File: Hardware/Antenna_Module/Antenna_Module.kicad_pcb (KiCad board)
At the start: 2 copper layers, 80 x 80 mm, 18 parts, among them J1 Conn_Coaxial, J2 Conn_01x02_Pin, U1 X3C14P1-03S-1, U2 X3C14P1-03S-1, U3 TFM.120A

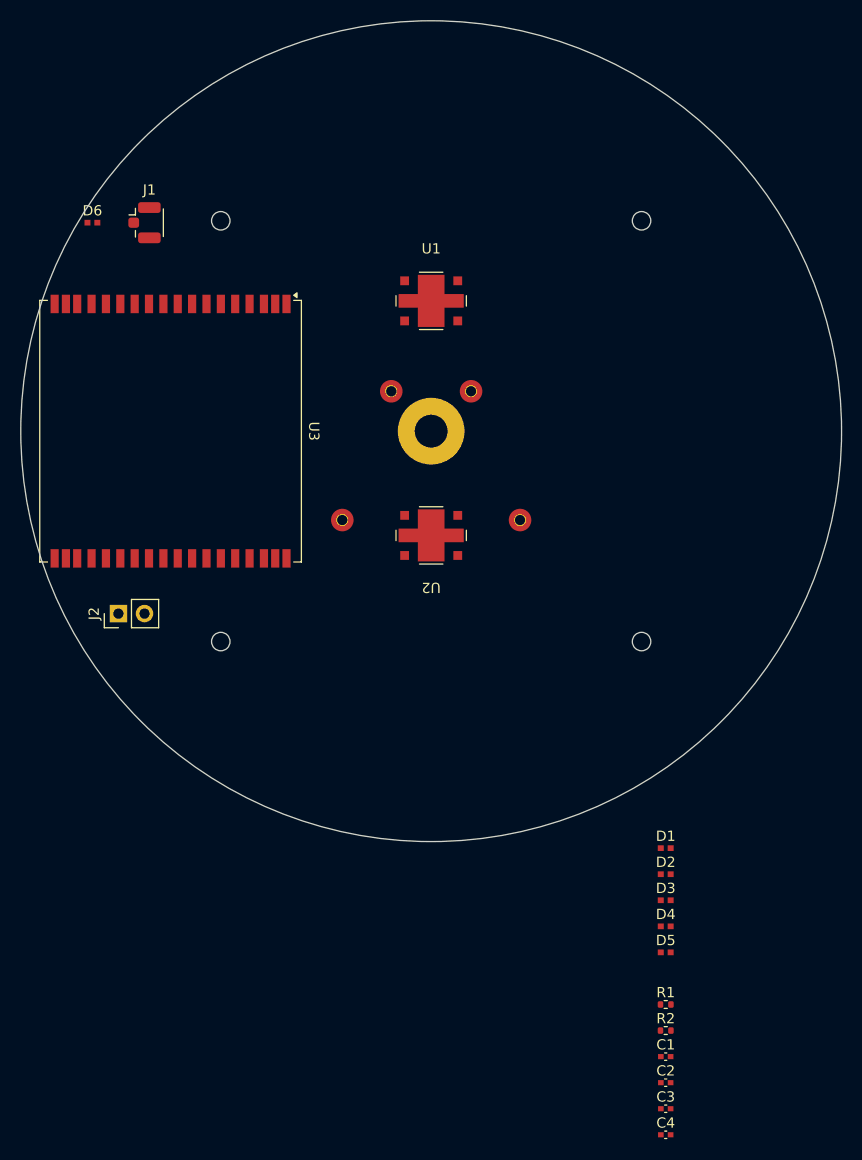
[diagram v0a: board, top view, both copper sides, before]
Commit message: 配線
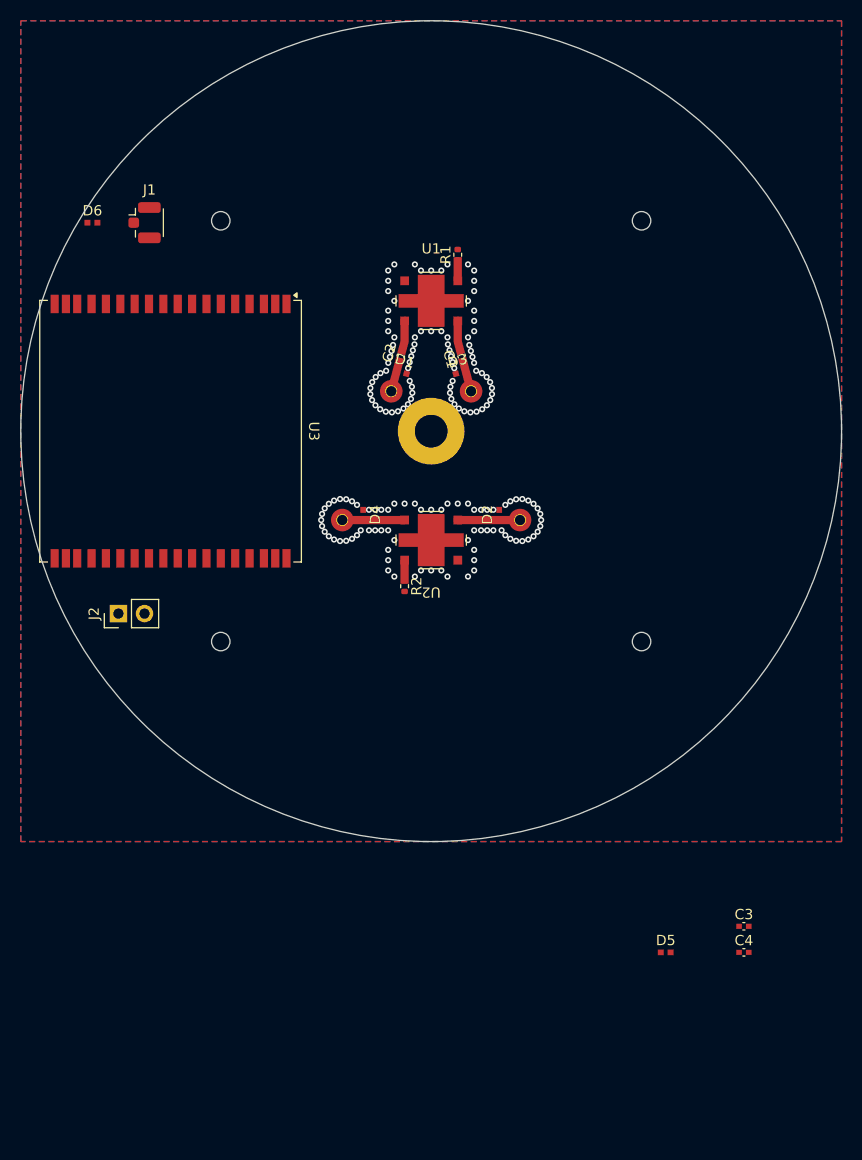
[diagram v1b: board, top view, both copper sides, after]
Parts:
- moved R1 75.8 mm to (2.59, -17.2), turned to 90 degrees
- moved C2 75.4 mm to (-2.97, -7.32), turned to 75 degrees
- moved C1 71.1 mm to (2.97, -7.32), turned to 105 degrees
- moved D3 55.2 mm to (2.87, -5.72), turned to 15 degrees
- moved D1 53.0 mm to (-2.87, -5.72), turned to -15 degrees
- moved R2 50.2 mm to (-2.59, 15.1), turned to -90 degrees
- moved D4 49.8 mm to (-6.63, 8.15), turned to -90 degrees
- moved D2 38.6 mm to (6.63, 8.15), turned to 90 degrees
- moved C3 19.3 mm to (30.5, 48.3)
- moved C4 19.3 mm to (30.5, 50.8)
- moved U2 0.46 mm to (0.00, 10.6)
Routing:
- net Net-(AE1B-LB2): track 0.00 -> 6.07 mm
- net Net-(AE1B-LB1): track 0.00 -> 6.07 mm
- net Net-(U1-∠θ-90): track 0.00 -> 2.01 mm
- net Net-(U1-∠θ): track 0.00 -> 2.01 mm
- net GND: vias 0 -> 158
- added copper zone on B.Cu, net GND
- added copper zone on F.Cu, net GND
